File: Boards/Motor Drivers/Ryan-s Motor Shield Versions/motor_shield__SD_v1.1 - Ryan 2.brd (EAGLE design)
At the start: 77.1 x 52.1 mm, 25 parts

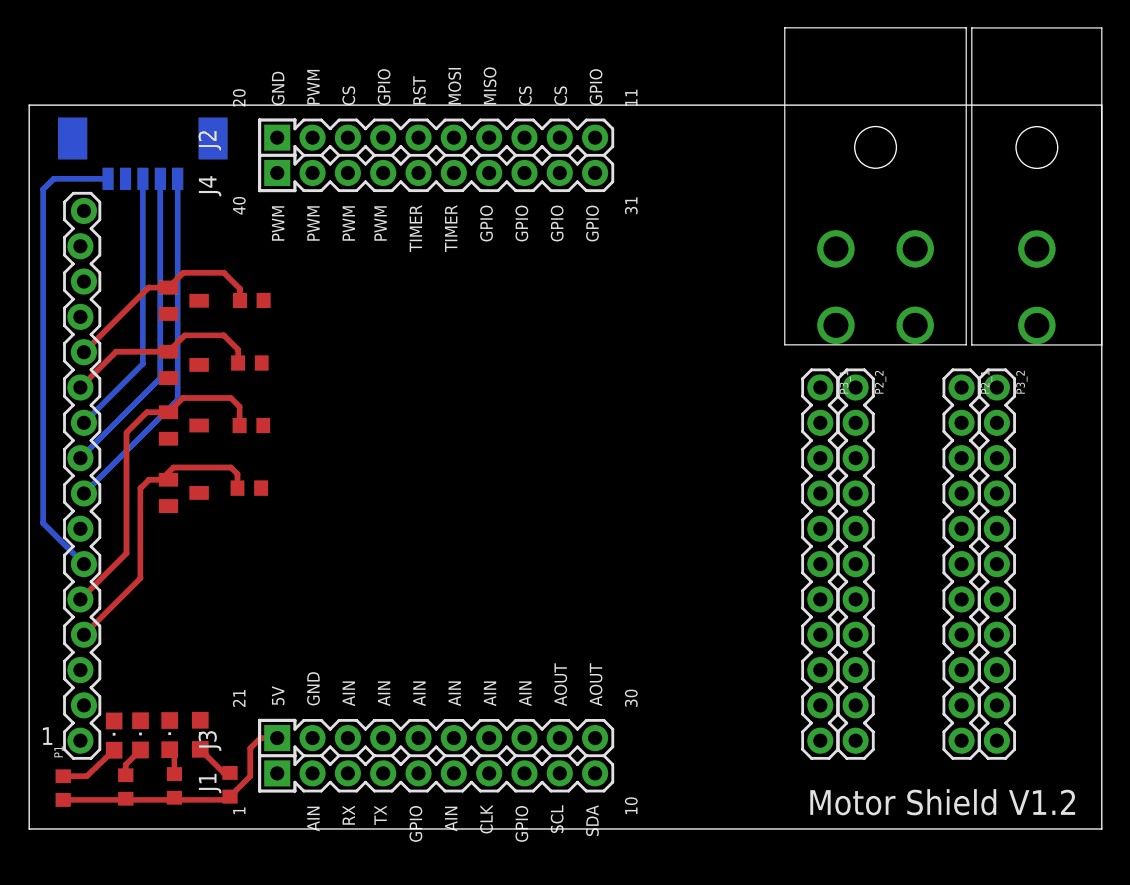
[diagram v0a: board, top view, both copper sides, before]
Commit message: Completed Routing
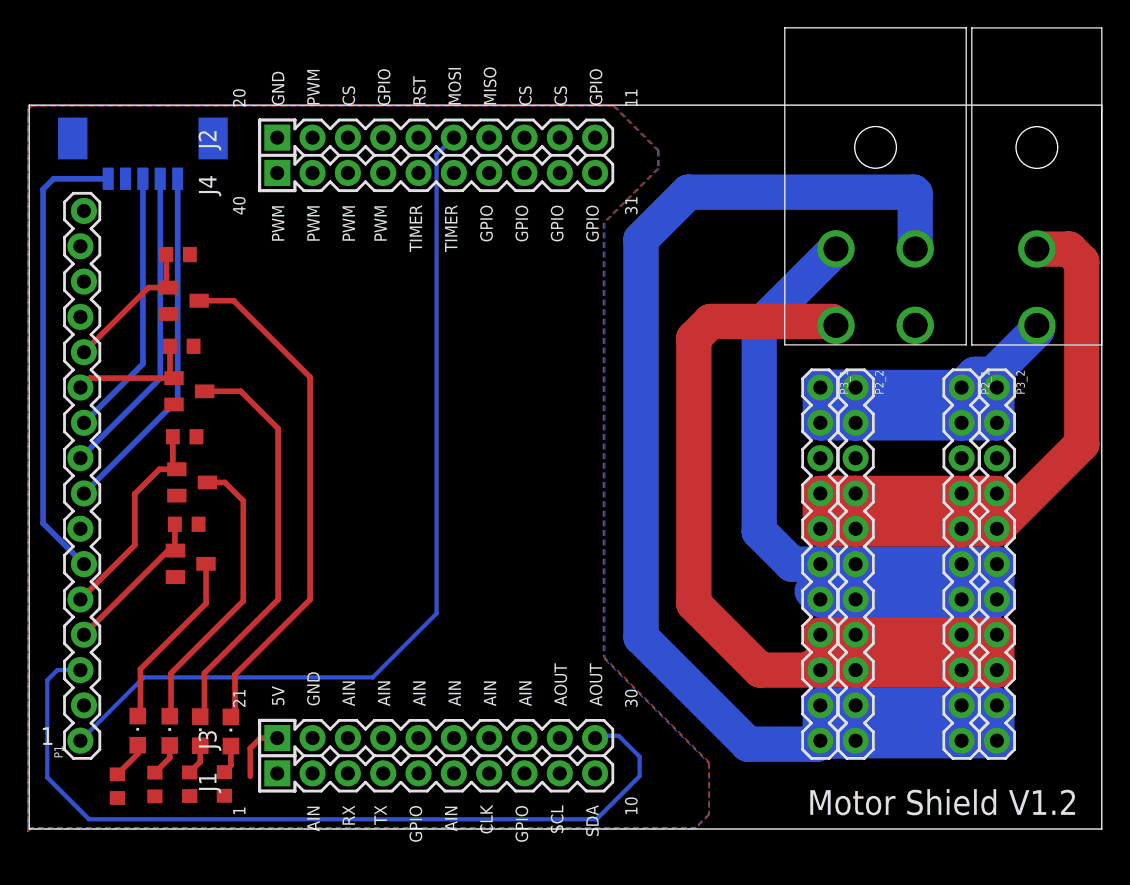
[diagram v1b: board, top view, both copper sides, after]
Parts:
- moved R3 11.6 mm to (14.0, 3.24)
- moved LED3 8.41 mm to (14.5, 7.01)
- moved R1 8.10 mm to (6.34, 3.08)
- moved R6 6.24 mm to (10.7, 41.3)
- moved R5 5.20 mm to (11.3, 21.9)
- moved MN1 5.12 mm to (11.6, 19.1)
- moved R8 5.04 mm to (11.0, 34.7)
- moved R7 4.87 mm to (11.2, 28.2)
- moved R2 4.60 mm to (11.5, 3.22)
- moved LED1 4.51 mm to (7.81, 7.07)
- moved LED2 4.31 mm to (12.3, 7.03)
- moved MN4 4.14 mm to (11.7, 24.9)
- moved MN2 1.94 mm to (11.5, 31.5)
- moved R4 1.40 mm to (9.04, 3.20)
- moved LED4 0.30 mm to (10.1, 7.05)
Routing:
- net MOTOR_A: track 0.00 -> 110.6 mm
- net MOTOR_B: track 0.00 -> 74.5 mm
- net MOTOR_C: track 0.00 -> 68.2 mm
- net PWR_GND: track 0.00 -> 64.5 mm
- net PWM: track 0.00 -> 64.2 mm
- net DIRECTION: track 0.00 -> 60.1 mm
- net HIGH_VOL: track 0.00 -> 43.0 mm
- net N$30: track 0.00 -> 37.1 mm
- net N$16: track 0.00 -> 29.4 mm
- net N$41: track 0.00 -> 20.8 mm
- net +5V: track 18.4 -> 4.26 mm
- net N$15: track 0.00 -> 13.0 mm
- net CURRENT_MONITOR: track 21.5 -> 11.1 mm
- net *INHIBIT: track 24.1 -> 15.4 mm
- net CURRENT_REF: track 14.3 -> 9.42 mm
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- added copper zone on layer 1, net GND
- added copper zone on layer 16, net GND
